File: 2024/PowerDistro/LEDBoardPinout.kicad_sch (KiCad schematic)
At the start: 33 parts, among them U1 PCA9685

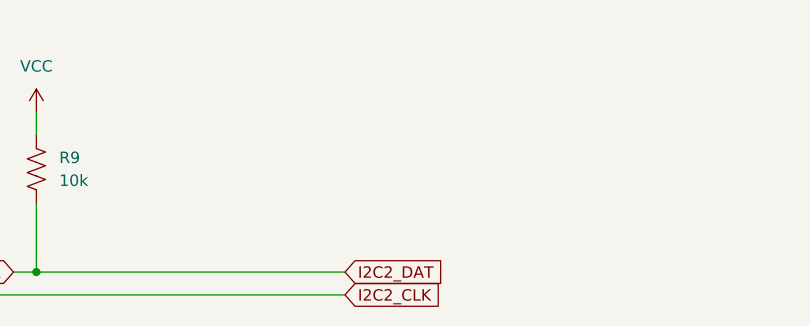
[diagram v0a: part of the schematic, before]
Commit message: Release
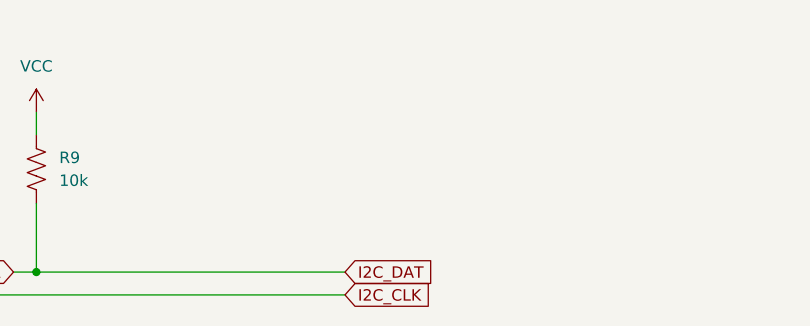
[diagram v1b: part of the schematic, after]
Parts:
- C1: footprint Capacitor_SMD:C_0603_1608Metric -> Capacitor_SMD:C_1206_3216Metric
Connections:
- net I2C2_CLK renamed I2C_CLK
- net I2C2_DAT renamed I2C_DAT
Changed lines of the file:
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@@
 		)
 	)
-	(global_label "I2C2_CLK"
+	(global_label "I2C_CLK"
 		(shape input)
 		(at 127 161.29 0)
@@
 		)
 		(property "Intersheetrefs" "${INTERSHEET_REFS}"
-			(at 138.8147 161.29 0)
+			(at 137.6052 161.29 0)
 			(effects
 				(font
@@
 		)
 	)
-	(global_label "I2C2_DAT"
+	(global_label "I2C_DAT"
 		(shape input)
 		(at 127 158.75 0)
@@
 		)
 		(property "Intersheetrefs" "${INTERSHEET_REFS}"
-			(at 138.5728 158.75 0)
+			(at 137.3633 158.75 0)
 			(effects
 				(font
@@
 			)
 		)
-		(property "Footprint" "Capacitor_SMD:C_0603_1608Metric"
+		(property "Footprint" "Capacitor_SMD:C_1206_3216Metric"
 			(at 152.0952 85.09 0)
 			(effects
